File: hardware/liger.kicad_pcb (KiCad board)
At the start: 2 copper layers, 33.1 x 92.2 mm, 56 parts, among them J1 Conn_02x08_Odd_Even, Q1 Q_NPN_BEC, Q4 PMOS-DMG3413L, U1 ESP-WROOM-32, U10 EKMC1601112, U12 soft-button-4x, U2 IR-RX-TSOP34438, U3 SPH0645LM4H-B, U4 MCP73831T, U5 MAX98357AETE+T, U6 SI7020-A20, U8 TSL45315CL, U9 AP2112

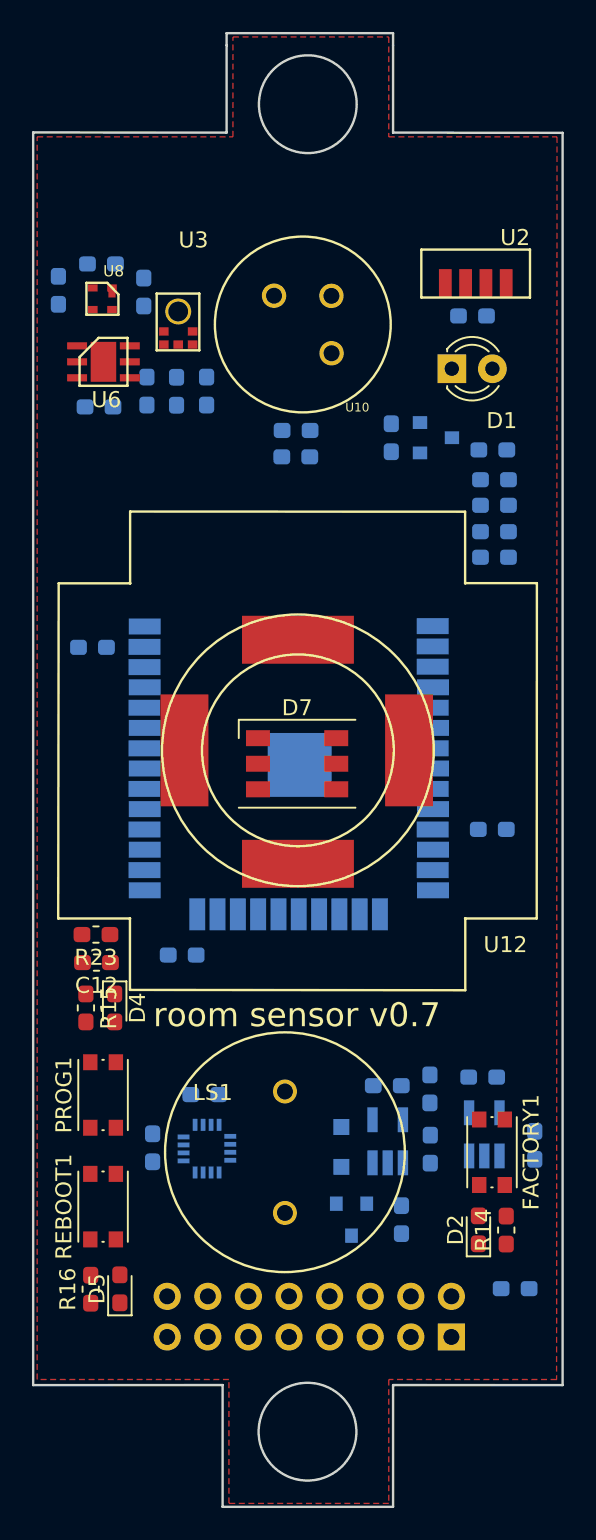
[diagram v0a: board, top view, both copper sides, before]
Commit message: corrections
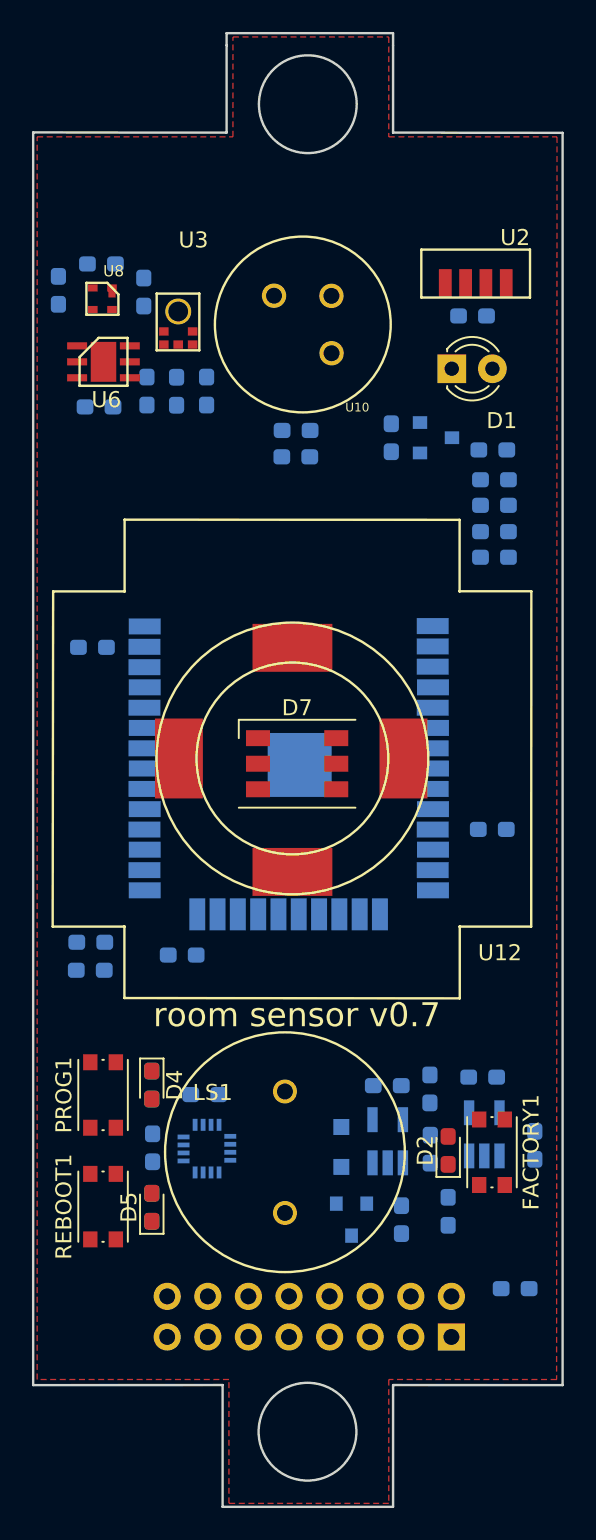
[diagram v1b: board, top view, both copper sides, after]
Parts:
- C12, R14, R15, R16, R23: moved to B.Cu
- moved R16 6.39 mm to (137.9, 116.5)
- moved R15 6.35 mm to (137.9, 108.8)
- moved D5 5.48 mm to (137.9, 116.5)
- moved D4 5.35 mm to (137.9, 108.8)
- moved D2 5.32 mm to (156.5, 112.9)
- moved R14 3.82 mm to (156.5, 116.7), turned to 270 degrees
- moved C12 0.62 mm to (134.1, 101.6), turned to 0 degrees
- moved U12 0.61 mm to (146.7, 88.4)
- moved R23 0.58 mm to (134.1, 99.9), turned to 0 degrees
